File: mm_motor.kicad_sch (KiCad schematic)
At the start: 2 parts, among them J2 Conn_01x06_Pin, M1 N20_encoder

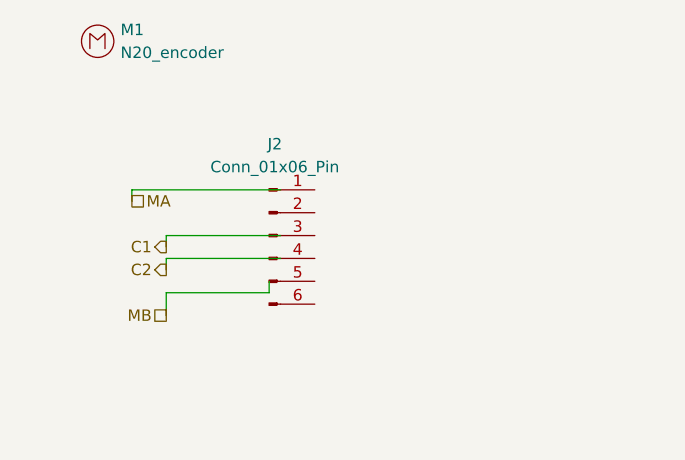
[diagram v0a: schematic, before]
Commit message: TP3
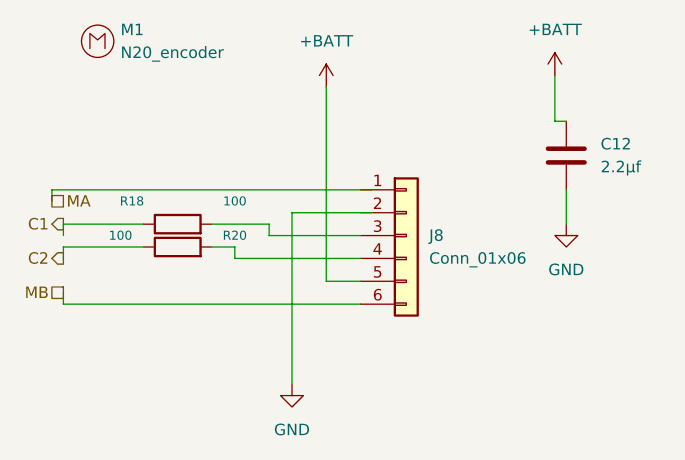
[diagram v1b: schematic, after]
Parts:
- removed J2: Conn_01x06_Pin, symbol Connector:Conn_01x06_Pin
- added C12: 2.2µf, Capacitor_SMD:C_0603_1608Metric, symbol Device:C
- added J8: Conn_01x06, Connector_PinHeader_2.54mm:PinHeader_1x06_P2.54mm_Vertical, symbol Connector_Generic:Conn_01x06
- added R18, R20: 100, Resistor_SMD:R_0603_1608Metric, symbol Device:R
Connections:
- net C1: now also R18.1
- net C2: now also R20.1
- net MB: now also J8.6 (Pin_6)
- new net: J8.4 (Pin_4), R20.2
- new net: J8.3 (Pin_3), R18.2
- new net +BATT: C12.1, J8.5 (Pin_5)
- new net GND: C12.2
